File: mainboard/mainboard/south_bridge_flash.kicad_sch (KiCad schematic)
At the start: 4 parts, among them U1 GD25D05CT

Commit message: working on new pcb
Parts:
- C402: footprint Capacitor_SMD:C_0603_1608Metric_Pad1.08x0.95mm_HandSolder -> Capacitor_SMD:C_0402_1005Metric_Pad0.74x0.62mm_HandSolder
- R404: footprint Resistor_SMD:R_0603_1608Metric_Pad0.98x0.95mm_HandSolder -> Resistor_SMD:R_0402_1005Metric_Pad0.72x0.64mm_HandSolder
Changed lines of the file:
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@@
       (effects (font (size 1.27 1.27)) (justify left))
     )
-    (property "Footprint" "Capacitor_SMD:C_0603_1608Metric_Pad1.08x0.95mm_HandSolder" (at 169.8752 88.9 0)
+    (property "Footprint" "Capacitor_SMD:C_0402_1005Metric_Pad0.74x0.62mm_HandSolder" (at 169.8752 88.9 0)
       (effects (font (size 1.27 1.27)) hide)
     )
@@
       (project "mainboard"
         (path "/e63e39d7-6ac0-4ffd-8aa3-1841a4541b55/90a5bc85-07ac-4ee1-af41-887c984cc4b9"
-          (reference "C402") (unit 1) (value "100n") (footprint "Capacitor_SMD:C_0603_1608Metric_Pad1.08x0.95mm_HandSolder")
+          (reference "C402") (unit 1) (value "100n") (footprint "Capacitor_SMD:C_0402_1005Metric_Pad0.74x0.62mm_HandSolder")
         )
         (path "/e63e39d7-6ac0-4ffd-8aa3-1841a4541b55/ee636c63-5fee-42d9-b500-aef9f04ef5c4"
-          (reference "C402") (unit 1) (value "100n") (footprint "Capacitor_SMD:C_0603_1608Metric_Pad1.08x0.95mm_HandSolder")
+          (reference "C402") (unit 1) (value "100n") (footprint "Capacitor_SMD:C_0402_1005Metric_Pad0.74x0.62mm_HandSolder")
         )
         (path "/e63e39d7-6ac0-4ffd-8aa3-1841a4541b55/ee636c63-5fee-42d9-b500-aef9f04ef5c4/e539fd0d-6f44-42c6-b17c-465bf8b74b11"
-          (reference "C402") (unit 1) (value "100n") (footprint "Capacitor_SMD:C_0603_1608Metric_Pad1.08x0.95mm_HandSolder")
+          (reference "C75") (unit 1) (value "100n") (footprint "Capacitor_SMD:C_0402_1005Metric_Pad0.74x0.62mm_HandSolder")
         )
       )
@@
       (effects (font (size 1.27 1.27)) (justify right))
     )
-    (property "Footprint" "Resistor_SMD:R_0603_1608Metric_Pad0.98x0.95mm_HandSolder" (at 138.938 86.36 90)
+    (property "Footprint" "Resistor_SMD:R_0402_1005Metric_Pad0.72x0.64mm_HandSolder" (at 138.938 86.36 90)
       (effects (font (size 1.27 1.27)) hide)
     )
@@
       (project "mainboard"
         (path "/e63e39d7-6ac0-4ffd-8aa3-1841a4541b55/90a5bc85-07ac-4ee1-af41-887c984cc4b9"
-          (reference "R404") (unit 1) (value "10k") (footprint "Resistor_SMD:R_0603_1608Metric_Pad0.98x0.95mm_HandSolder")
+          (reference "R404") (unit 1) (value "10k") (footprint "Resistor_SMD:R_0402_1005Metric_Pad0.72x0.64mm_HandSolder")
         )
         (path "/e63e39d7-6ac0-4ffd-8aa3-1841a4541b55/ee636c63-5fee-42d9-b500-aef9f04ef5c4"
-          (reference "R404") (unit 1) (value "10k") (footprint "Resistor_SMD:R_0603_1608Metric_Pad0.98x0.95mm_HandSolder")
+          (reference "R404") (unit 1) (value "10k") (footprint "Resistor_SMD:R_0402_1005Metric_Pad0.72x0.64mm_HandSolder")
         )
         (path "/e63e39d7-6ac0-4ffd-8aa3-1841a4541b55/ee636c63-5fee-42d9-b500-aef9f04ef5c4/e539fd0d-6f44-42c6-b17c-465bf8b74b11"
-          (reference "R404") (unit 1) (value "10k") (footprint "Resistor_SMD:R_0603_1608Metric_Pad0.98x0.95mm_HandSolder")
+          (reference "R17") (unit 1) (value "10k") (footprint "Resistor_SMD:R_0402_1005Metric_Pad0.72x0.64mm_HandSolder")
         )
       )
@@
       (effects (font (size 1.27 1.27)) (justify right))
     )
-    (property "Footprint" "Resistor_SMD:R_0603_1608Metric_Pad0.98x0.95mm_HandSolder" (at 130.048 86.36 90)
+    (property "Footprint" "Resistor_SMD:R_0402_1005Metric_Pad0.72x0.64mm_HandSolder" (at 130.048 86.36 90)
       (effects (font (size 1.27 1.27)) hide)
     )
@@
       (project "mainboard"
         (path "/e63e39d7-6ac0-4ffd-8aa3-1841a4541b55/90a5bc85-07ac-4ee1-af41-887c984cc4b9"
-          (reference "R404") (unit 1) (value "10k") (footprint "Resistor_SMD:R_0603_1608Metric_Pad0.98x0.95mm_HandSolder")
+          (reference "R404") (unit 1) (value "10k") (footprint "Resistor_SMD:R_0402_1005Metric_Pad0.72x0.64mm_HandSolder")
         )
         (path "/e63e39d7-6ac0-4ffd-8aa3-1841a4541b55/ee636c63-5fee-42d9-b500-aef9f04ef5c4"
-          (reference "R405") (unit 1) (value "10k") (footprint "Resistor_SMD:R_0603_1608Metric_Pad0.98x0.95mm_HandSolder")
+          (reference "R405") (unit 1) (value "10k") (footprint "Resistor_SMD:R_0402_1005Metric_Pad0.72x0.64mm_HandSolder")
         )
         (path "/e63e39d7-6ac0-4ffd-8aa3-1841a4541b55/ee636c63-5fee-42d9-b500-aef9f04ef5c4/e539fd0d-6f44-42c6-b17c-465bf8b74b11"
-          (reference "R403") (unit 1) (value "10k") (footprint "Resistor_SMD:R_0603_1608Metric_Pad0.98x0.95mm_HandSolder")
+          (reference "R16") (unit 1) (value "10k") (footprint "Resistor_SMD:R_0402_1005Metric_Pad0.72x0.64mm_HandSolder")
         )
       )
@@
         )
         (path "/e63e39d7-6ac0-4ffd-8aa3-1841a4541b55/ee636c63-5fee-42d9-b500-aef9f04ef5c4/e539fd0d-6f44-42c6-b17c-465bf8b74b11"
-          (reference "U1") (unit 1) (value "GD25D05CT") (footprint "Package_SO:SOP-8_3.9x4.9mm_P1.27mm")
+          (reference "U10") (unit 1) (value "GD25D05CT") (footprint "Package_SO:SOP-8_3.9x4.9mm_P1.27mm")
         )
       )

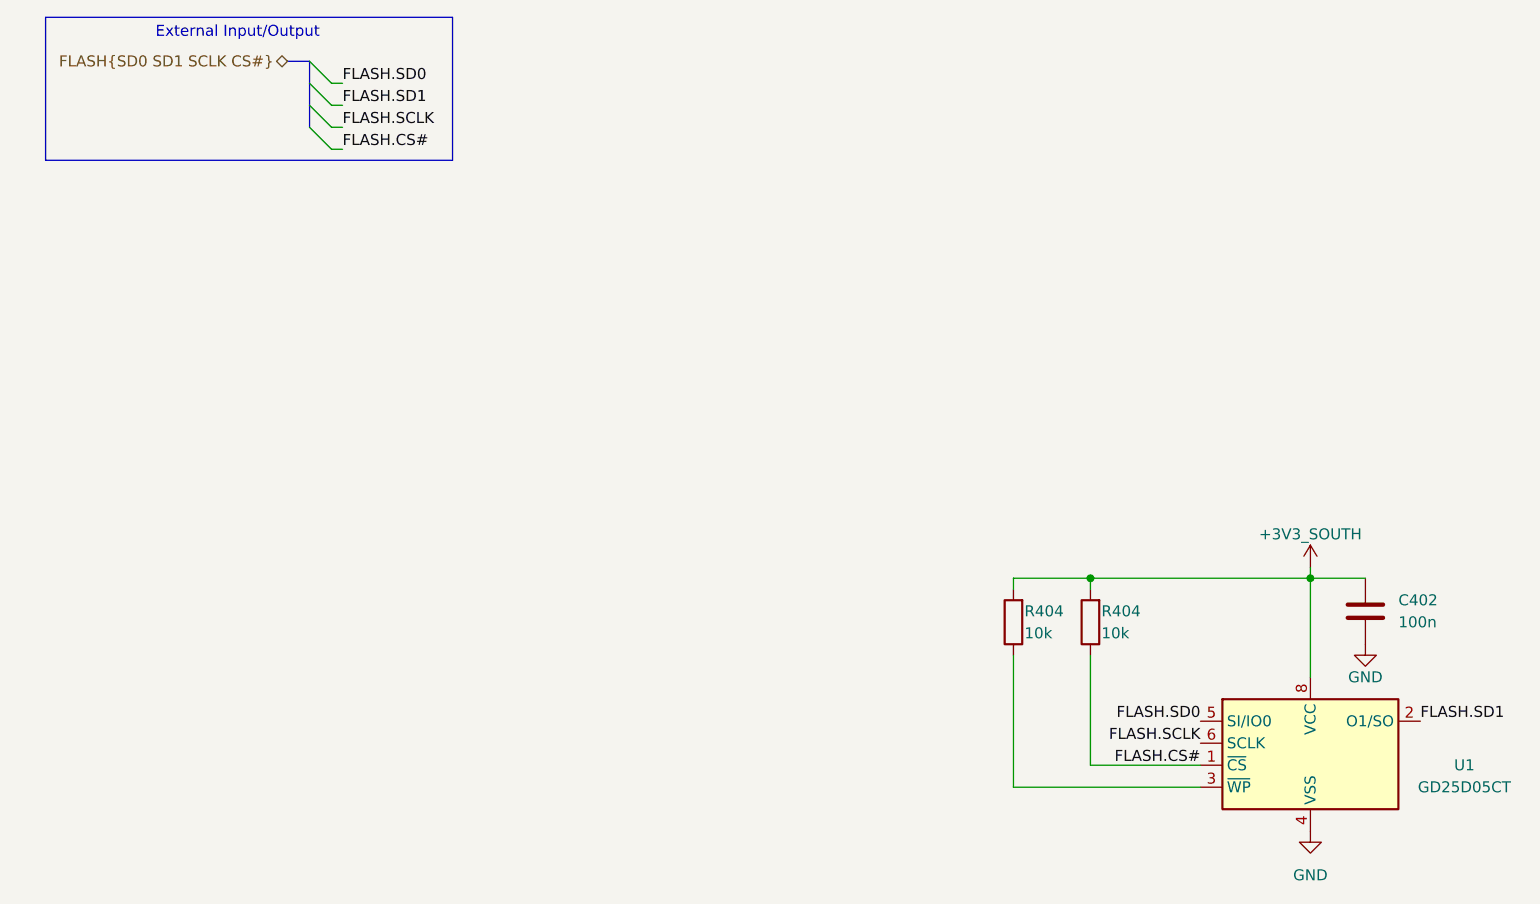
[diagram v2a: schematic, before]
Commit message: version 1.0
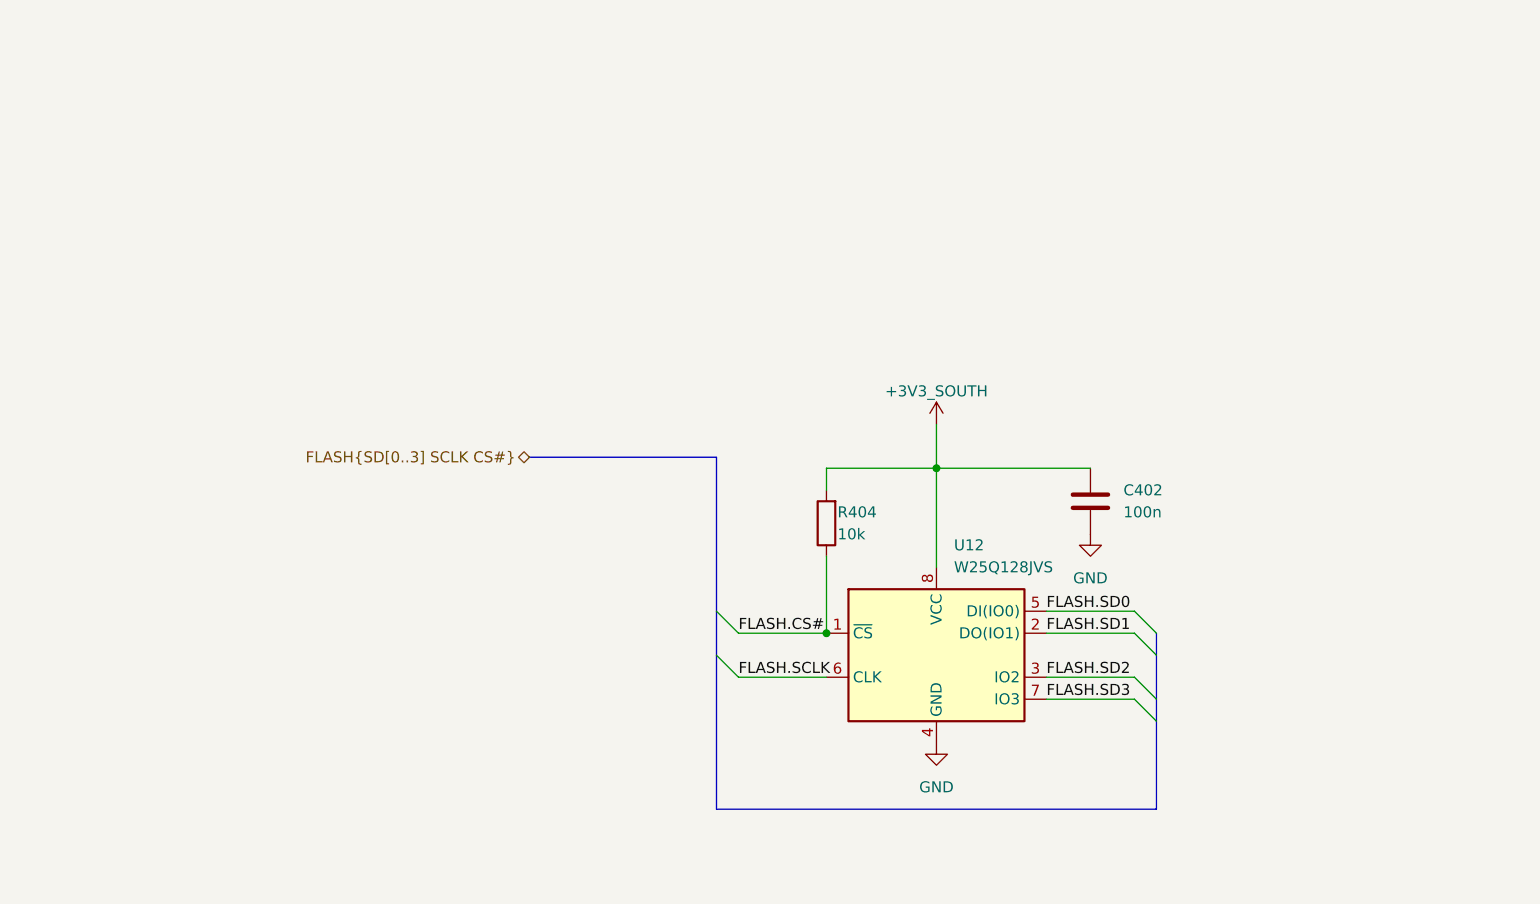
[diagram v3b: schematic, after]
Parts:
- removed R404 (x2): 10k, Resistor_SMD:R_0402_1005Metric_Pad0.72x0.64mm_HandSolder, symbol Device:R
- removed U1: GD25D05CT, Package_SO:SOP-8_3.9x4.9mm_P1.27mm, symbol Memory_Flash:GD25D05CT
- added R404: 10k, Resistor_SMD:R_0402_1005Metric_Pad0.72x0.64mm_HandSolder, symbol Device:R
- added U12: W25Q128JVS, Package_SO:SOIC-8_5.23x5.23mm_P1.27mm, symbol Memory_Flash:W25Q128JVS
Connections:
- net +3V3_SOUTH: now also R404.2, U12.8 (VCC)
- net FLASH.CS#: now also R404.1, U12.1 (~{CS})
- net FLASH.SCLK: now also U12.6 (CLK)
- net FLASH.SD0: now also U12.5 (DI(IO0))
- net FLASH.SD1: now also U12.2 (DO(IO1))
- net GND: now also U12.4 (GND)
- new net FLASH.SD2: U12.3 (IO2)
- new net FLASH.SD3: U12.7 (IO3)
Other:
- note removed: "External Input/Output"
